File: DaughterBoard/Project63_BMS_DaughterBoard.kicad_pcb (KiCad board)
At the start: 4 copper layers, 166 parts, among them J1 430450200, J4 1-794106-0, J5 430450200, Q1 ZXTN4004KTC, U1 BQ79614PAPRQ1

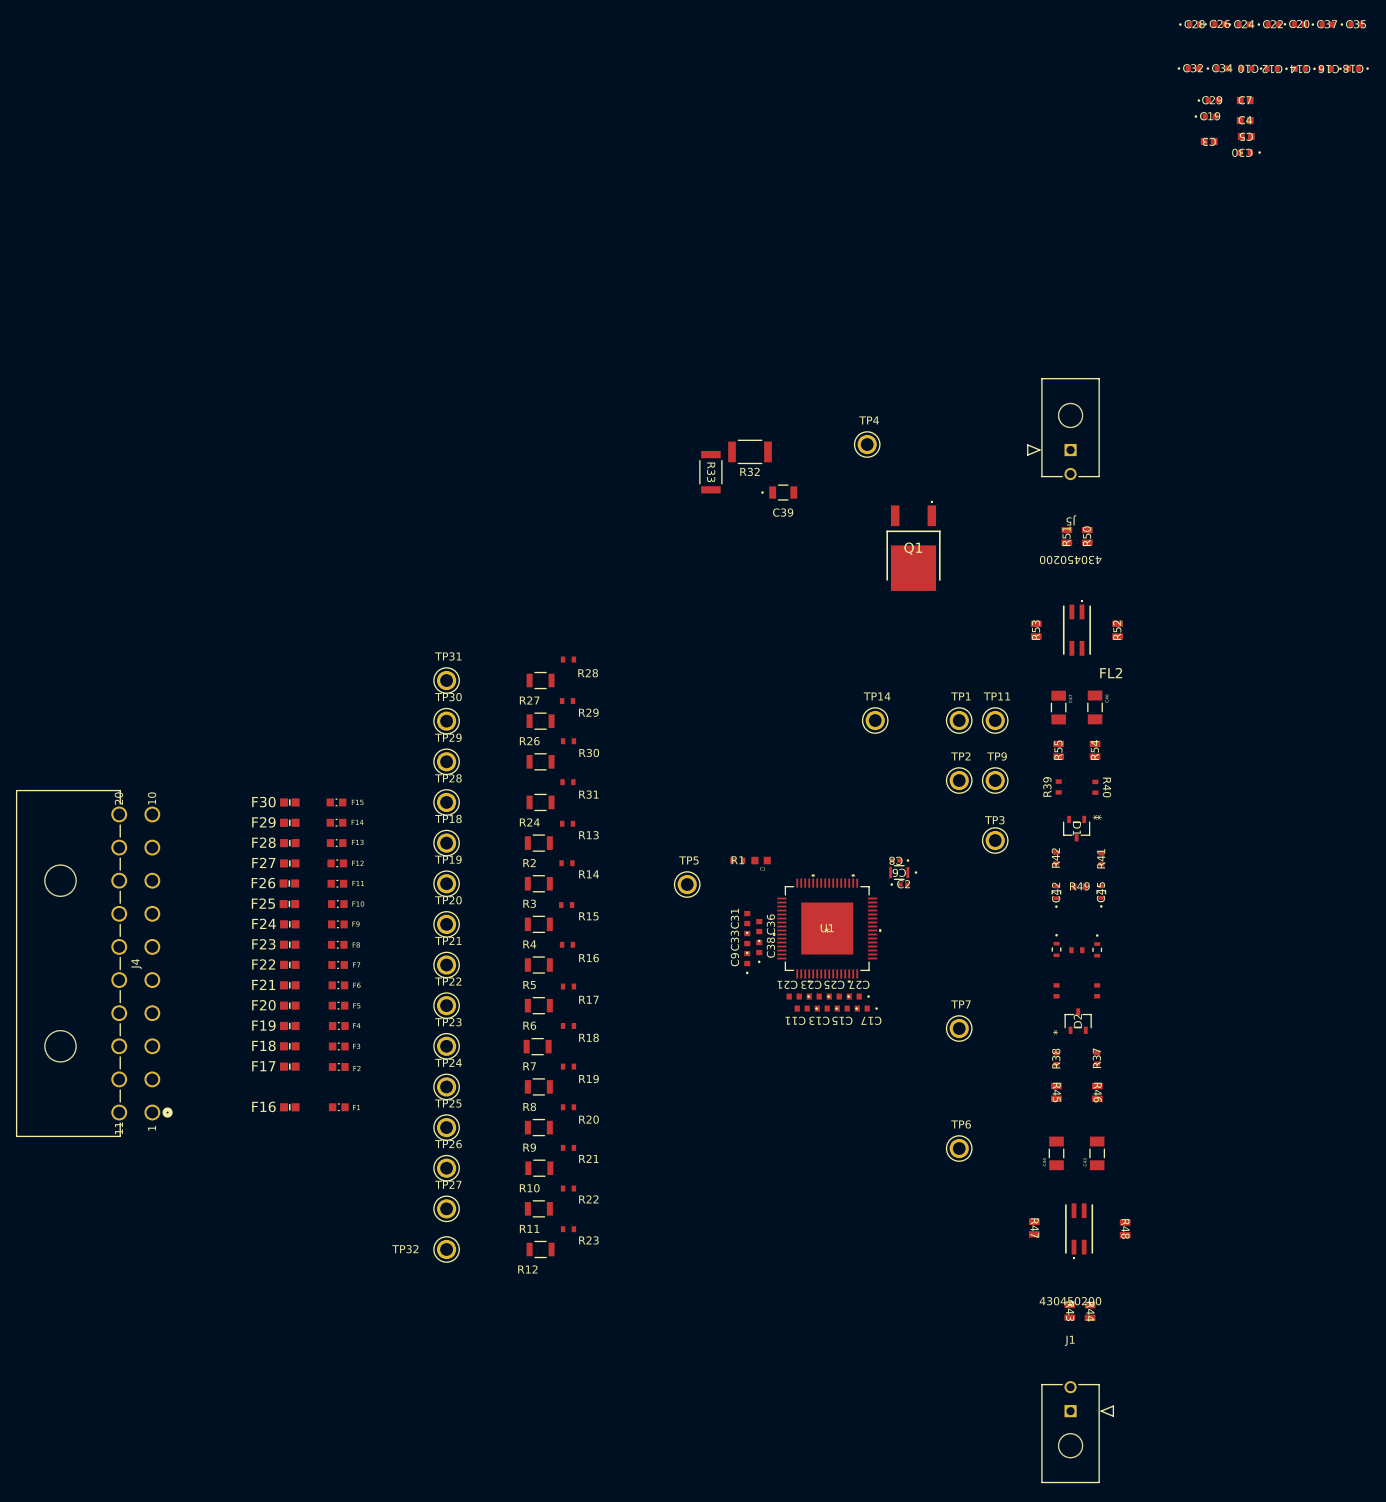
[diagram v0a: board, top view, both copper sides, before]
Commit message: layout
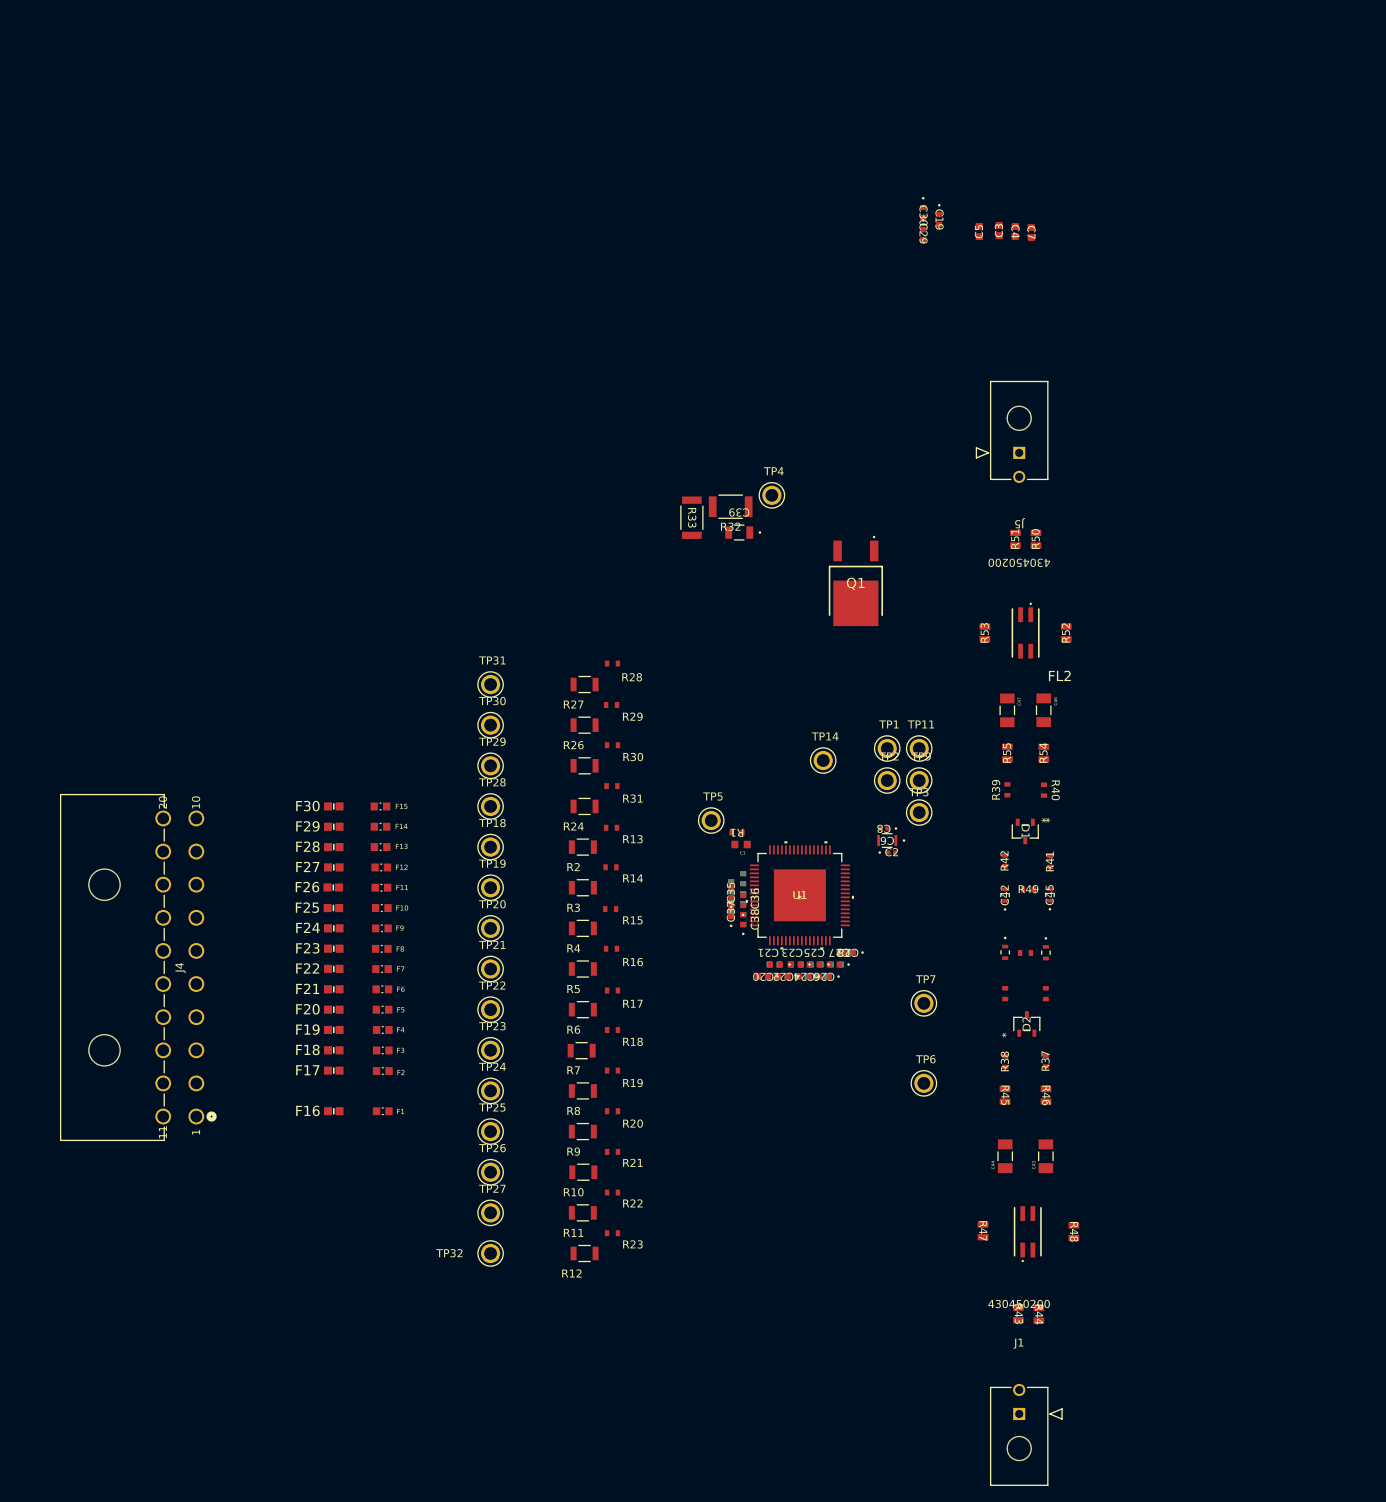
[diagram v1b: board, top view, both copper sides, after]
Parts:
- C10, C11, C12, C13, C14, C15, C16, C17, C18, C31, C32, C33, C34, C9: moved to B.Cu
- moved C20 136.6 mm to (161.5, 100.5), turned to 180 degrees
- moved C22 133.8 mm to (164.0, 100.5), turned to 180 degrees
- moved C35 133.7 mm to (157.5, 90.0), turned to 90 degrees
- moved C37 133.6 mm to (157.5, 92.4), turned to 90 degrees
- moved C24 131.1 mm to (166.6, 100.5), turned to 180 degrees
- moved C16 129.8 mm to (168.7, 100.5), turned to 0 degrees
- moved C14 129.4 mm to (166.4, 100.5), turned to 0 degrees
- moved C12 128.9 mm to (163.9, 100.5), turned to 0 degrees
- moved C26 128.9 mm to (169.1, 100.5), turned to 180 degrees
- moved C10 128.6 mm to (161.5, 100.5), turned to 0 degrees
- moved C18 127.5 mm to (171.6, 97.5), turned to 0 degrees
- moved C28 123.8 mm to (172.1, 97.5), turned to 180 degrees
- moved C34 121.4 mm to (157.5, 91.8), turned to 90 degrees
- moved C32 117.5 mm to (157.5, 89.3), turned to 90 degrees
- moved C30 40.9 mm to (181.5, 5.00), turned to -90 degrees
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
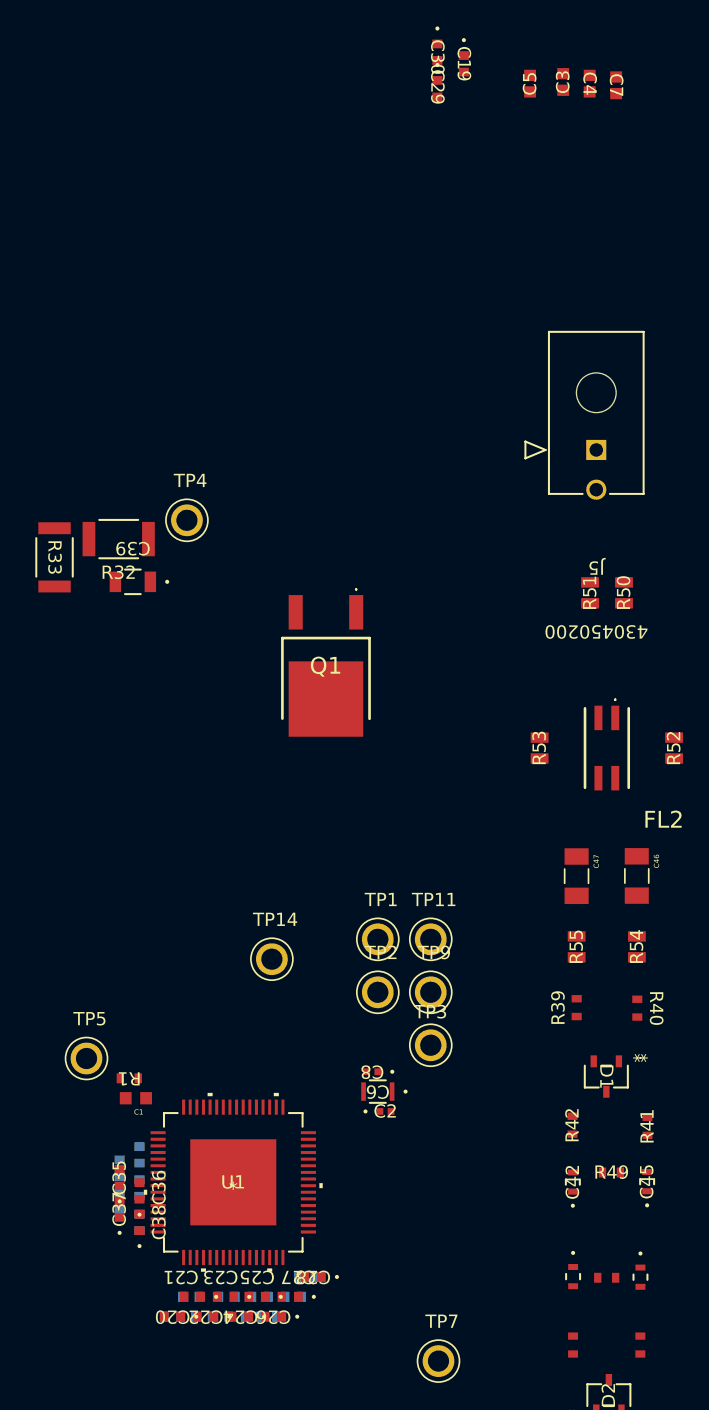
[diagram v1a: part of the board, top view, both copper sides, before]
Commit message: done
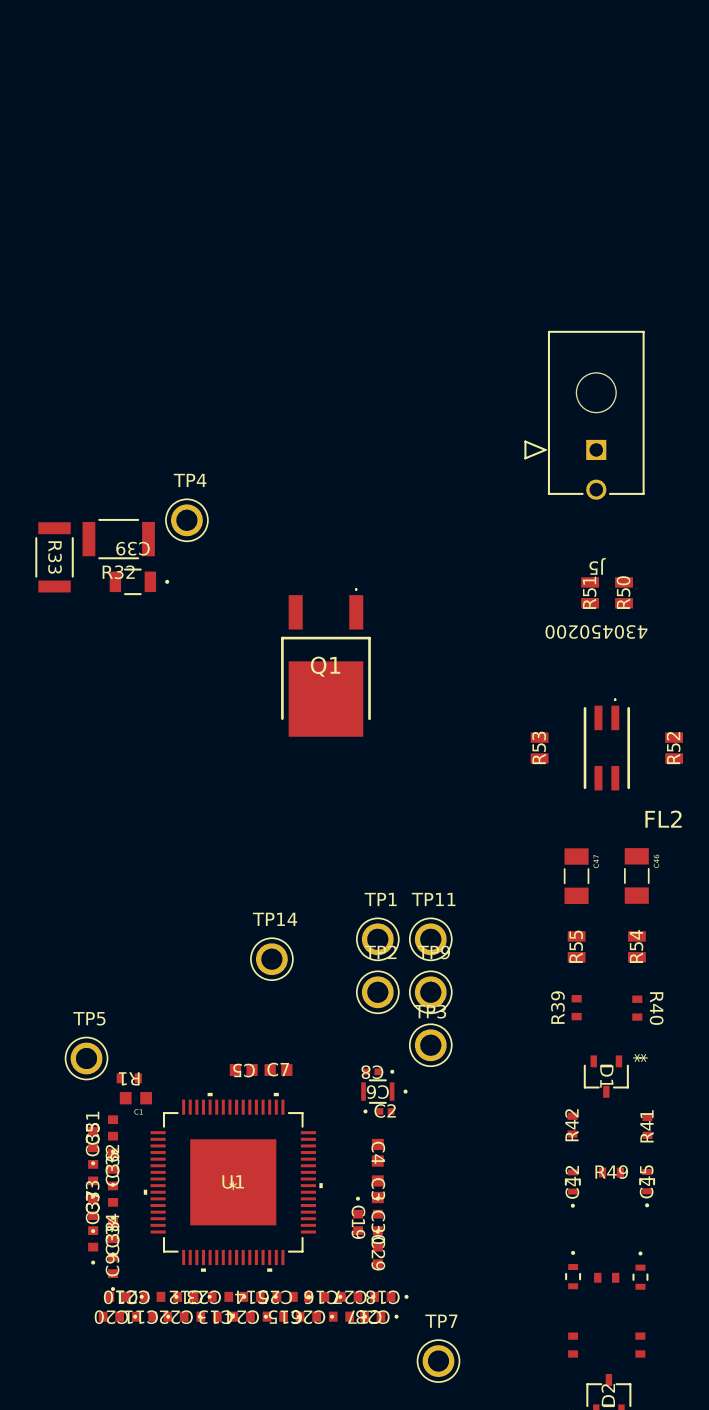
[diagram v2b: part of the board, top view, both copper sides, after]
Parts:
- C10, C11, C12, C13, C14, C15, C16, C17, C18, C31, C32, C33, C34, C9: moved to F.Cu
- moved C30 88.5 mm to (177.0, 93.4)
- moved C29 88.2 mm to (177.0, 95.9)
- moved C19 87.9 mm to (175.5, 93.4)
- moved C3 84.8 mm to (177.0, 90.9), turned to -90 degrees
- moved C4 82.3 mm to (177.0, 88.1)
- moved C7 78.6 mm to (169.5, 81.9), turned to 0 degrees
- moved C5 77.6 mm to (166.9, 81.9), turned to 180 degrees
- moved C18 5.95 mm to (177.4, 99.0), turned to 180 degrees
- moved C28 5.41 mm to (176.6, 100.5)
- moved C20 4.62 mm to (156.9, 100.5)
- moved C10 4.38 mm to (157.4, 99.0), turned to 180 degrees
- moved C17 4.26 mm to (174.9, 99.0), turned to 180 degrees
- moved C27 4.16 mm to (174.3, 100.5)
- moved C16 3.94 mm to (172.4, 99.0), turned to 180 degrees
- moved C21 3.92 mm to (159.4, 100.5)
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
